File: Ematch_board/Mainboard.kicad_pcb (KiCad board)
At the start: 4 copper layers, 57 x 53 mm, 124 parts, among them J1 Conn_01x02_Male, J10 Conn_01x02_Male, J11 Conn_Coaxial, J2 Conn_01x02_Male, J3 Conn_01x02_Male, J4 Conn_01x02_Male, J5 Conn_01x02_Male, J6 Conn_01x02_Male, J7 RBUS, J8 USB_C_Receptacle_USB2.0, J9 Conn_01x02_Male, Q1 MMDT2222A, Q51 PMV20ENR, Q52 PMV20ENR, Q53 PMV20ENR, Q54 PMV20ENR, Q55 PMV20ENR, Q56 PMV20ENR, U1 LTV-247, U2 LTC4411, U3 SC4216H, U4 LTC4411, U5 SN65HVD230, U6 CP2102-GMR-QFN28

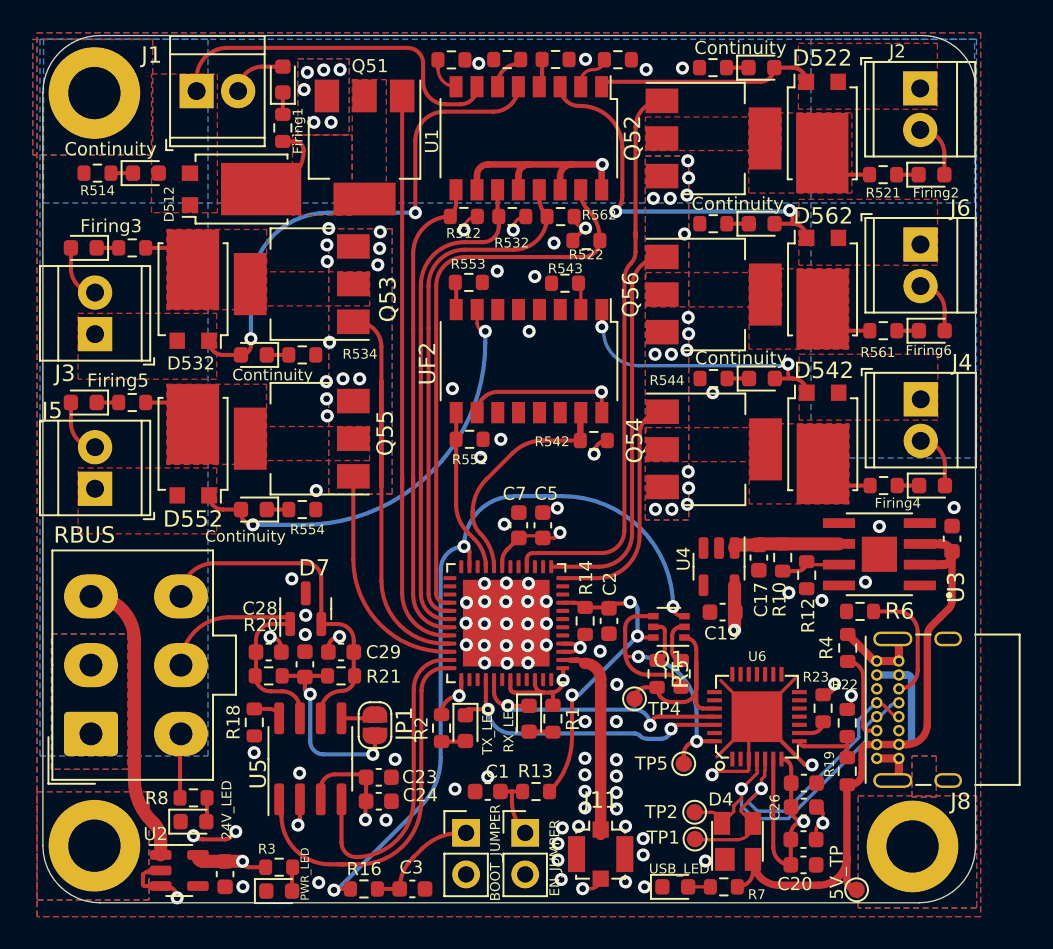
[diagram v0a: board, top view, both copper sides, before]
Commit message: DRC fixes
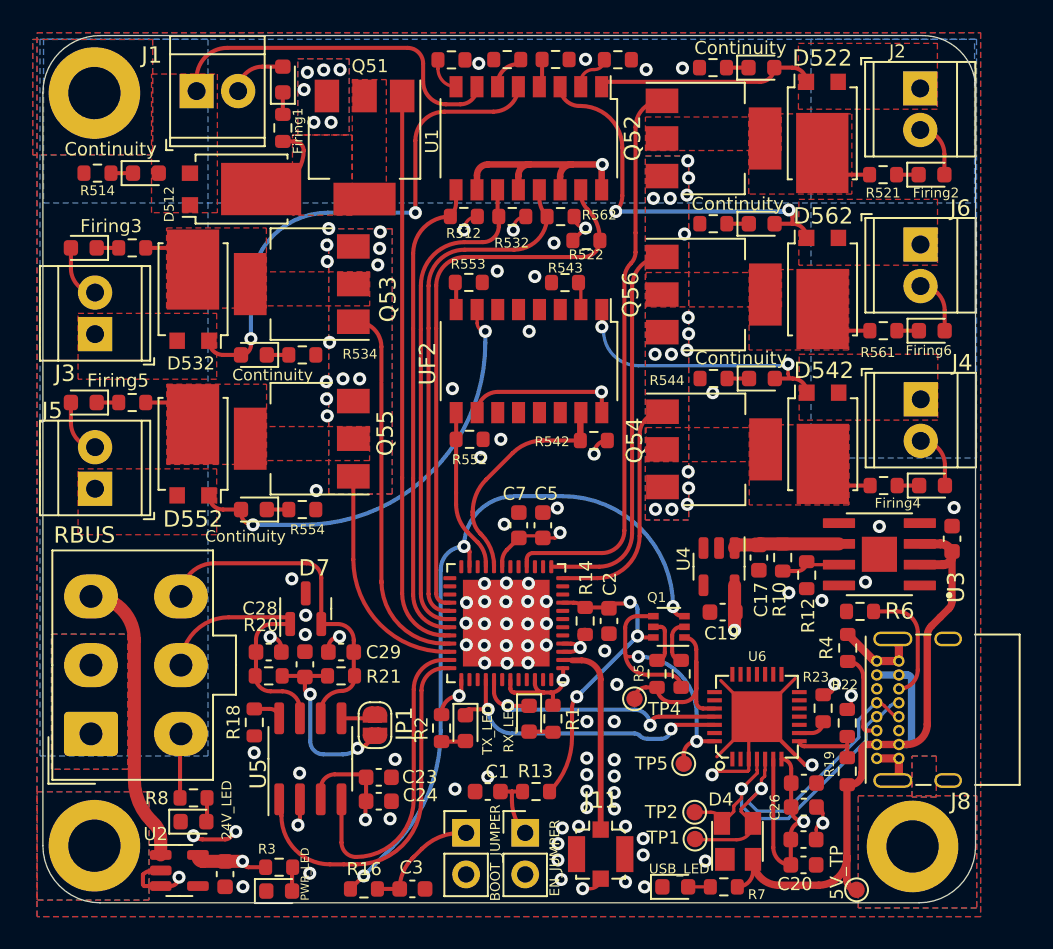
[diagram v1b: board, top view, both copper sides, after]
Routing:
- net /Nuke 3: track 29.5 -> 23.1 mm
- net /BOOT: track 45.8 -> 43.9 mm
- net Net-(D562-Pad1): track 23.8 -> 24.8 mm
- net Net-(C1-Pad1): track 4.84 -> 4.08 mm
- net /Vref: track 12.3 -> 11.6 mm
- net /Data+: track 21.9 -> 21.3 mm
- net Net-(R563-Pad1): track 2.05 -> 1.49 mm
